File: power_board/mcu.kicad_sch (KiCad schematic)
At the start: 12 parts, among them U1 STM32L431KCUx

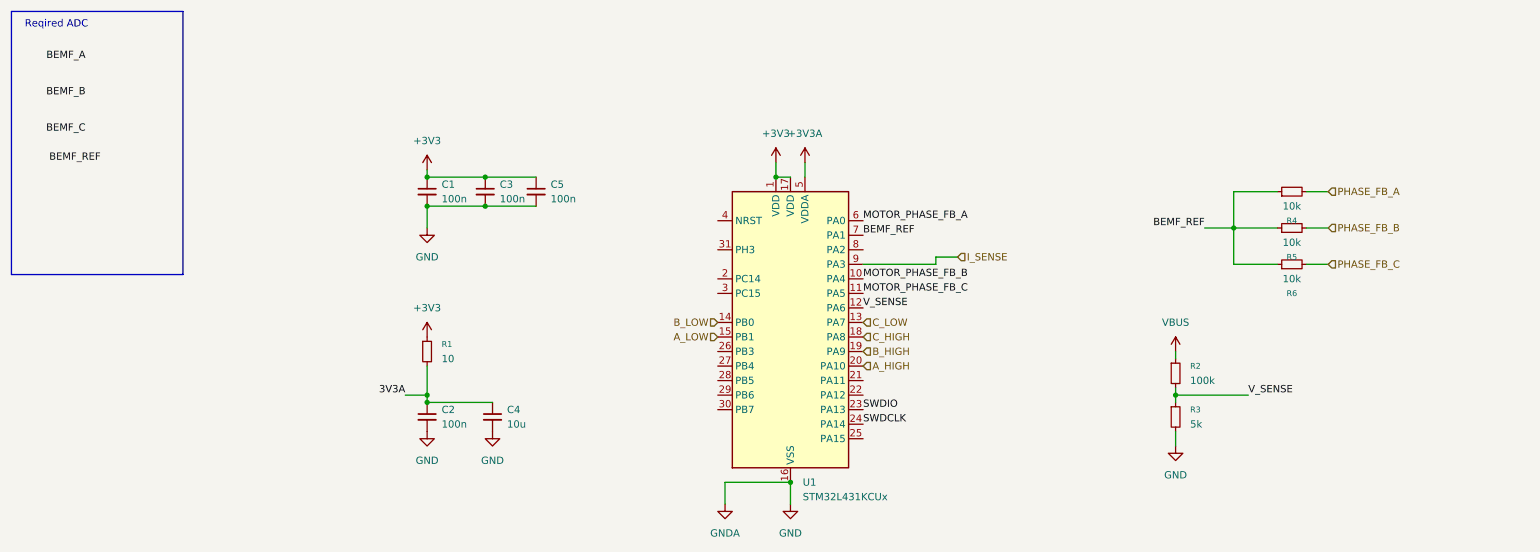
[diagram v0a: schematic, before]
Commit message: Start multichannel layout
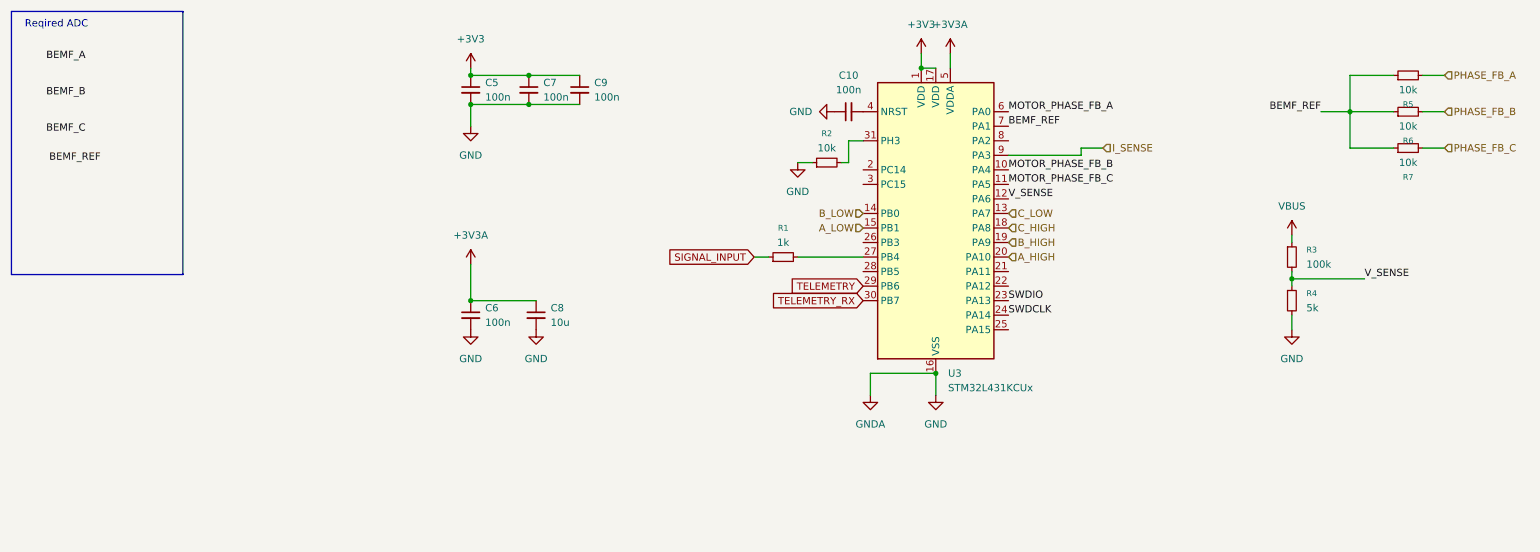
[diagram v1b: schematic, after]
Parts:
- added C10: 100n, Capacitor_SMD:C_0603_1608Metric, symbol Device:C_Small
- added R2: 10k, Resistor_SMD:R_0603_1608Metric, symbol Device:R_Small
- C5: renamed from C1; footprint (none) -> Capacitor_SMD:C_0603_1608Metric
- C6: renamed from C2; footprint (none) -> Capacitor_SMD:C_0603_1608Metric
- C7: renamed from C3; footprint (none) -> Capacitor_SMD:C_0603_1608Metric
- C8: renamed from C4; footprint (none) -> Capacitor_SMD:C_0603_1608Metric
- C9: renamed from C5; footprint (none) -> Capacitor_SMD:C_0603_1608Metric
- R1: value 10 -> 1k; footprint (none) -> Resistor_SMD:R_0603_1608Metric
- R3: renamed from R2; footprint (none) -> Resistor_SMD:R_0603_1608Metric
- R4: renamed from R3; footprint (none) -> Resistor_SMD:R_0603_1608Metric
- R5: renamed from R4; footprint (none) -> Resistor_SMD:R_0603_1608Metric
- R6: renamed from R5; footprint (none) -> Resistor_SMD:R_0603_1608Metric
- R7: renamed from R6; footprint (none) -> Resistor_SMD:R_0603_1608Metric
- renumbered U1 to U3
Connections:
- net +3V3: no longer R1.1
- net +3V3A: now also C6.1, C8.1
- net GND: now also C10.1, R2.1
- net at U3.27 (PB4): now also R1.2
- net TELEMETRY: now reaches U3.29 (PB6)
- net TELEMETRY_RX: now reaches U3.30 (PB7)
- net at U3.31 (PH3): now also R2.2
- net at U3.4 (NRST): now also C10.2
- removed net 3V3A: C6.1, C8.1, R1.2
- new net SIGNAL_INPUT: R1.1
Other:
- moved on the sheet: C5, C6, C7, C8, C9, R3, R4, R5, R6, R7, U3
